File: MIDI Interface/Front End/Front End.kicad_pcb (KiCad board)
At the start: 2 copper layers, 213 x 104.5 mm, 74 parts, among them J101 AudioJack2_SwitchT, J102 AudioJack2_SwitchT, J103 AudioJack2_SwitchT, J104 AudioJack2_SwitchT, J105 Conn_01x08, J106 AudioJack2_SwitchT, J107 AudioJack2_SwitchT, J108 AudioJack2_SwitchT, J109 AudioJack2_SwitchT, J110 Conn_02x08_Counter_Clockwise, J111 Conn_01x12, J112 AudioJack2_SwitchT, J113 AudioJack2_SwitchT, J114 AudioJack2_SwitchT, J115 AudioJack2_SwitchT, J116 AudioJack2_SwitchT, J117 Conn_01x08, J118 AudioJack2_SwitchT, J119 AudioJack2_SwitchT, J120 AudioJack2_SwitchT, J121 AudioJack2_SwitchT, J122 AudioJack2_SwitchT, J123 AudioJack2_SwitchT, J124 AudioJack2_SwitchT, J125 AudioJack2_SwitchT, J126 Conn_01x08, J127 AudioJack2_SwitchT, J128 AudioJack2_SwitchT, J129 AudioJack2_SwitchT, J130 AudioJack2_SwitchT, J131 AudioJack2_SwitchT, J132 AudioJack2_SwitchT, J133 AudioJack2_SwitchT, J134 AudioJack2_SwitchT, J135 Conn_01x08, J136 AudioJack2_SwitchT, J137 AudioJack2_SwitchT, J138 AudioJack2_SwitchT, J139 AudioJack2_SwitchT, SW101 SW_SPST, SW102 SW_SPST, SW103 SW_SPST, SW104 SW_SPST, U101 MOP-AL162A

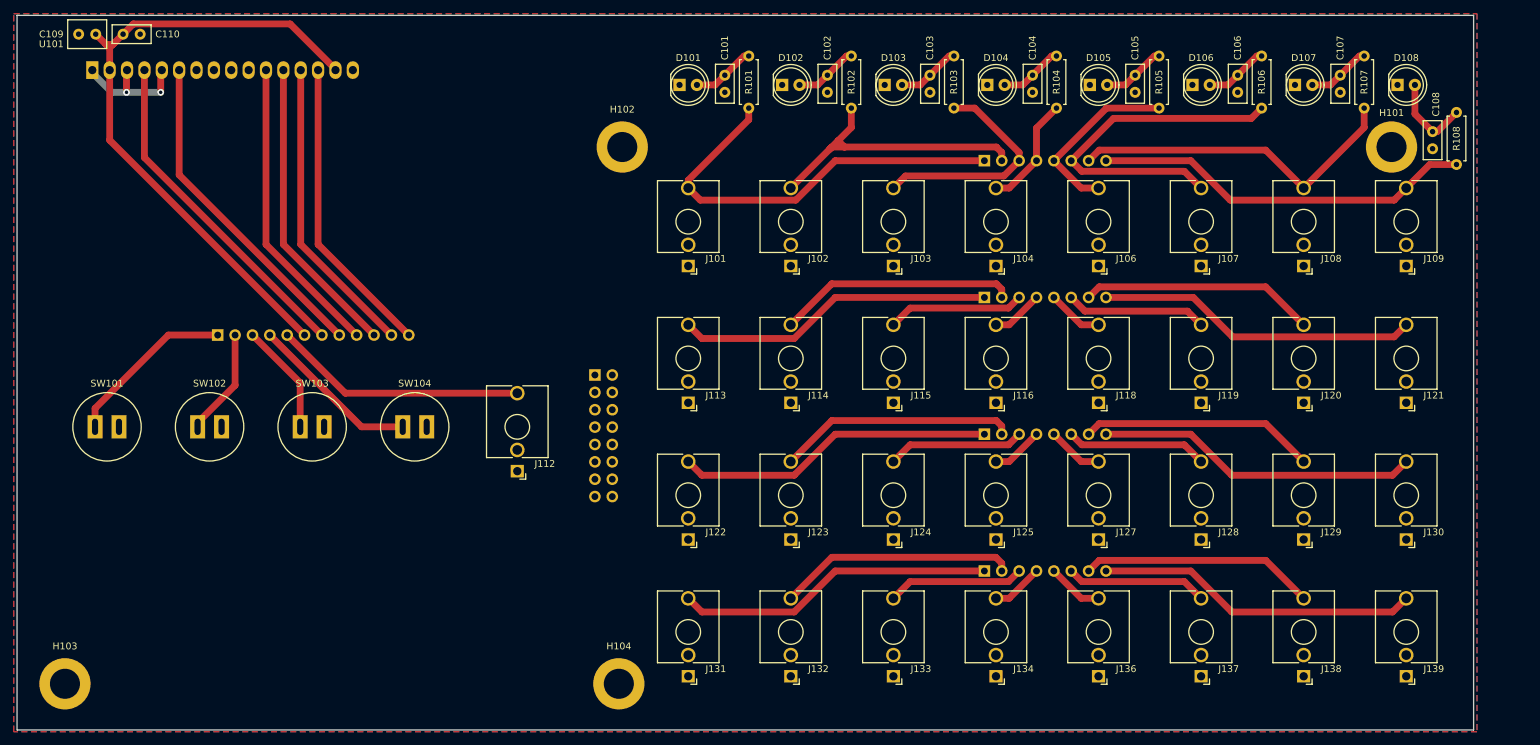
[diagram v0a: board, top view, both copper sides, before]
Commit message: New VCLPF and Out
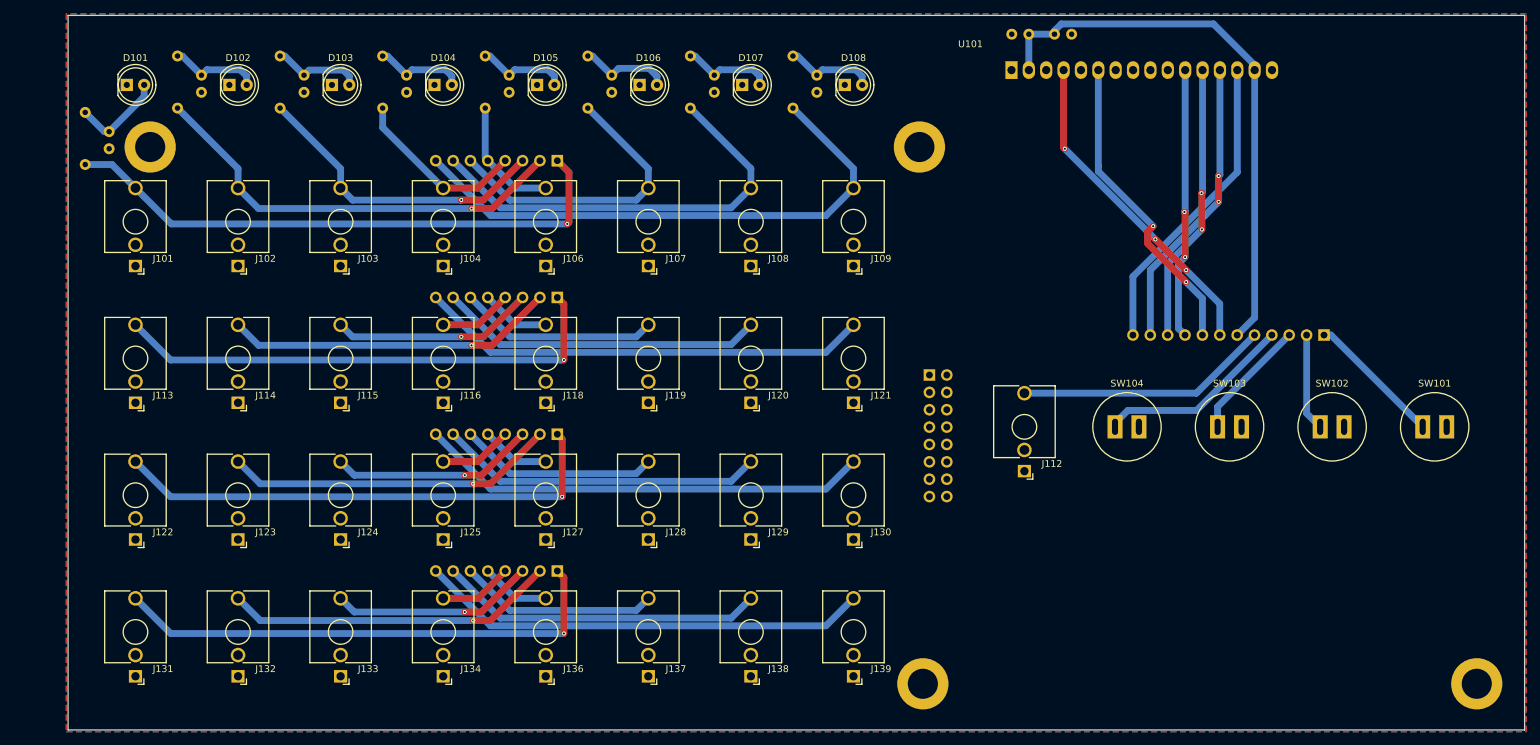
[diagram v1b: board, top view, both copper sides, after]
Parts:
- C101: renamed from C108; moved to B.Cu
- C102: renamed from C107; moved to B.Cu
- C103: renamed from C106; moved to B.Cu
- C104: renamed from C105; moved to B.Cu
- C105: renamed from C104; moved to B.Cu
- C106: renamed from C103; moved to B.Cu
- C107: renamed from C102; moved to B.Cu
- C108: renamed from C101; moved to B.Cu
- C109, C110, H101, H102, H103, H104: moved to B.Cu
- R101: renamed from R108; moved to B.Cu
- R102: renamed from R107; moved to B.Cu
- R103: renamed from R106; moved to B.Cu
- R104: renamed from R105; moved to B.Cu
- R105: renamed from R104; moved to B.Cu
- R106: renamed from R103; moved to B.Cu
- R107: renamed from R102; moved to B.Cu
- R108: renamed from R101; moved to B.Cu
- moved H103 206.5 mm to (258.0, 138.5), turned to 180 degrees
- moved R101 200.5 mm to (54.5, 62.6)
- moved SW101 194.2 mm to (251.8, 100.9)
- moved C101 193.5 mm to (58.0, 60.2)
- moved H101 181.5 mm to (64.0, 60.0), turned to 180 degrees
- moved R102 173.5 mm to (68.0, 54.3)
- moved C102 166.5 mm to (71.5, 52.0)
- moved SW102 164.2 mm to (236.8, 100.9)
- moved J111 161.8 mm to (235.6, 87.5), turned to 90 degrees
- moved R103 143.5 mm to (83.0, 54.3)
- moved C109 140.2 mm to (196.2, 43.5), turned to 0 degrees
- moved C103 136.5 mm to (86.5, 52.0)
- moved U101 134.4 mm to (189.9, 48.8)
- moved SW103 134.2 mm to (221.8, 100.9)
- moved C110 132.5 mm to (192.5, 43.5), turned to 180 degrees
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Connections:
- C101 pad 2: Net-(D108-A) -> Net-(D101-A)
- C102 pad 2: Net-(D107-A) -> Net-(D102-A)
- C103 pad 2: Net-(D106-A) -> Net-(D103-A)
- C104 pad 2: Net-(D105-A) -> Net-(D104-A)
- C105 pad 2: Net-(D104-A) -> Net-(D105-A)
- C106 pad 2: Net-(D103-A) -> Net-(D106-A)
- C107 pad 2: Net-(D102-A) -> Net-(D107-A)
- C108 pad 2: Net-(D101-A) -> Net-(D108-A)
- R101 pad 1: Net-(J105-Pin_8) -> Net-(J105-Pin_1)
- R101 pad 2: Net-(D108-A) -> Net-(D101-A)
- R102 pad 1: Net-(J105-Pin_7) -> Net-(J105-Pin_2)
- R102 pad 2: Net-(D107-A) -> Net-(D102-A)
- R103 pad 1: Net-(J105-Pin_6) -> Net-(J105-Pin_3)
- R103 pad 2: Net-(D106-A) -> Net-(D103-A)
- R104 pad 1: Net-(J105-Pin_5) -> Net-(J105-Pin_4)
- R104 pad 2: Net-(D105-A) -> Net-(D104-A)
- R105 pad 1: Net-(J105-Pin_4) -> Net-(J105-Pin_5)
- R105 pad 2: Net-(D104-A) -> Net-(D105-A)
- R106 pad 1: Net-(J105-Pin_3) -> Net-(J105-Pin_6)
- R106 pad 2: Net-(D103-A) -> Net-(D106-A)
- R107 pad 1: Net-(J105-Pin_2) -> Net-(J105-Pin_7)
- R107 pad 2: Net-(D102-A) -> Net-(D107-A)
- R108 pad 1: Net-(J105-Pin_1) -> Net-(J105-Pin_8)
- R108 pad 2: Net-(D101-A) -> Net-(D108-A)
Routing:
- net Net-(J117-Pin_1): track 46.6 -> 74.3 mm, vias 0 -> 1
- net Net-(J135-Pin_1): track 46.6 -> 74.3 mm, vias 0 -> 1
- net Net-(J126-Pin_1): track 46.6 -> 74.0 mm, vias 0 -> 1
- net Net-(J105-Pin_8): track 55.8 -> 81.4 mm
- net Net-(J105-Pin_1): track 61.8 -> 84.2 mm, vias 0 -> 1
- net Net-(J105-Pin_2): track 43.5 -> 63.6 mm, vias 0 -> 1
- net Net-(J117-Pin_8): track 47.0 -> 66.1 mm
- net Net-(J126-Pin_8): track 47.2 -> 66.1 mm
- net Net-(J135-Pin_8): track 47.2 -> 66.1 mm
- net GND: track 18.2 -> 0.00 mm, vias 2 -> 0
- net Net-(J135-Pin_2): track 34.8 -> 48.5 mm, vias 0 -> 1
- net Net-(J126-Pin_2): track 34.9 -> 48.5 mm, vias 0 -> 1
- net Net-(J117-Pin_2): track 34.9 -> 48.3 mm, vias 0 -> 1
- net Net-(J105-Pin_7): track 49.7 -> 63.0 mm
- net Net-(J135-Pin_7): track 34.4 -> 47.6 mm
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- added copper zone on F.Cu, net Chassis
- added copper zone on B.Cu, net GND
- removed copper zone on B.Cu, net Chassis
- removed copper zone on F.Cu, net GND
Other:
- board text added: "JLCJLCJLCJLC"
